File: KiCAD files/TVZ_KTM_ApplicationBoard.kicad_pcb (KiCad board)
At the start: 2 copper layers, 160 x 60 mm, 63 parts, among them SW1 EG1271A, SW2 EG1271A, SW3 EG1271A, SW4 EG1271A, U1 LM75B, U2 MCP2551-I-P, U3 MCP2551-I-P, U4 NUCLEO64-F446RE, U5 NUCLEO64-F446RE

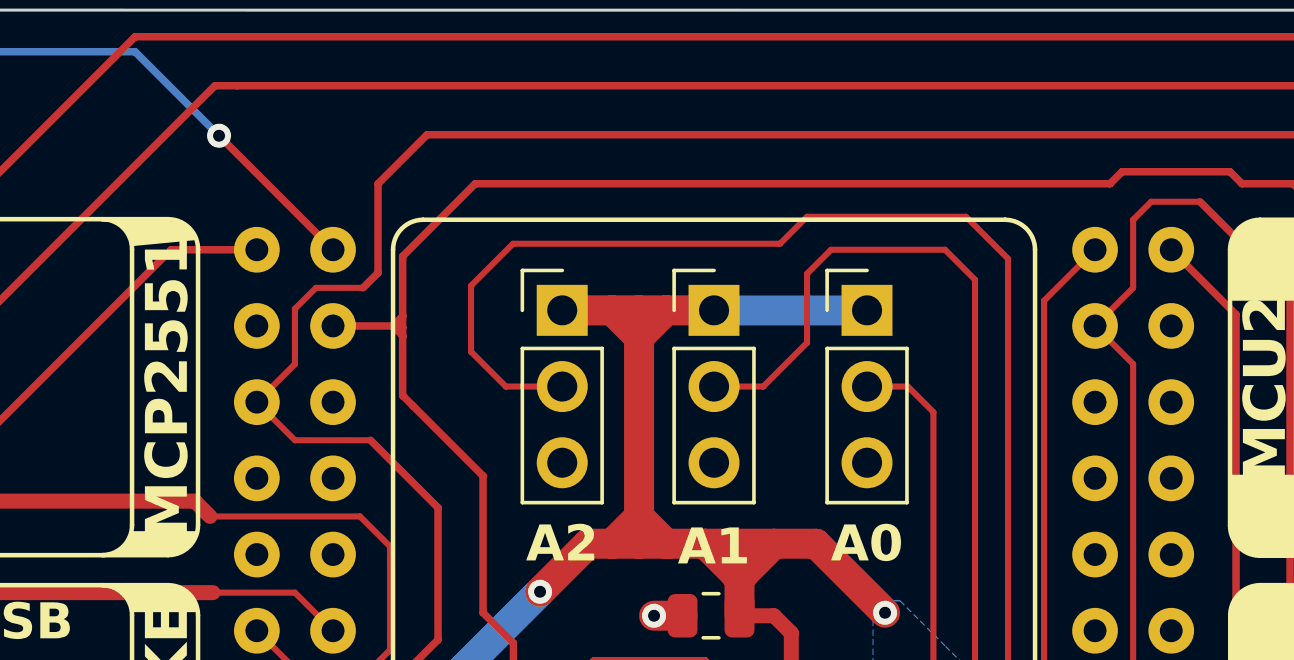
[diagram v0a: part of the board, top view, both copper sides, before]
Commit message: update
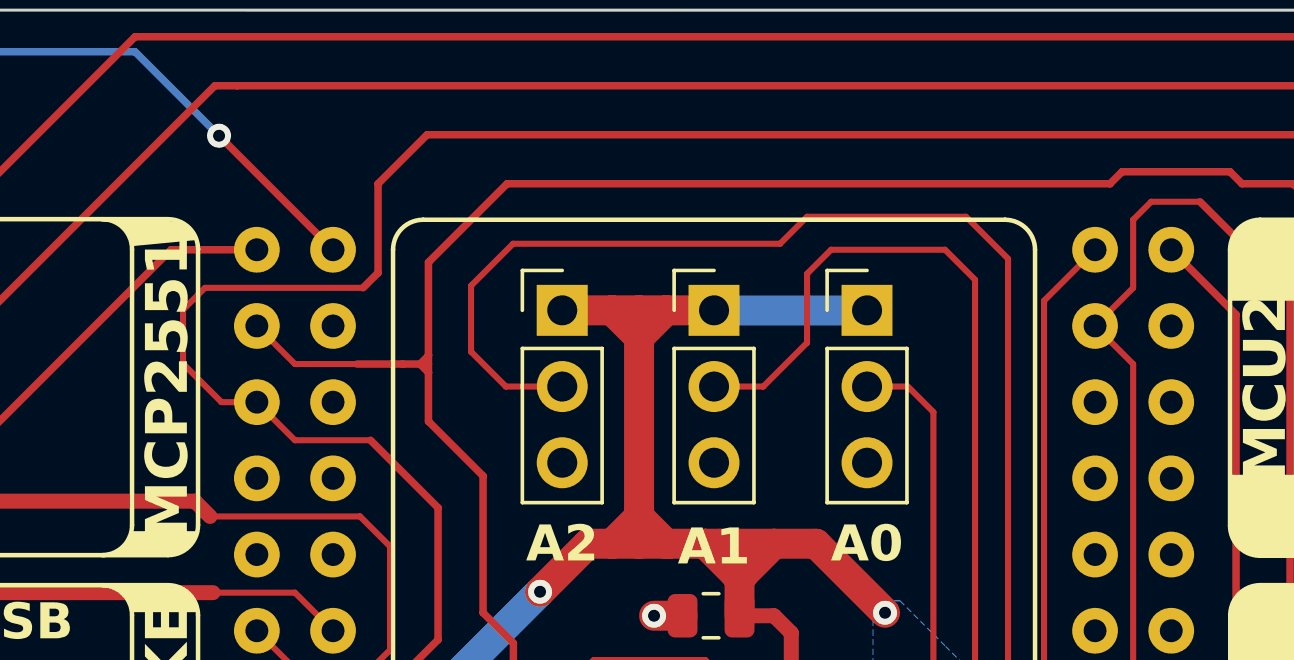
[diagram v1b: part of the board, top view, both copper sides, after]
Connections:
- U4 pad 41: unconnected-(U4-PB8-Pad41) -> I2C_SCL
- U4 pad 42: I2C_SCL -> unconnected-(U4-PC6-Pad42)
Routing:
- net I2C_SDA: track 150.3 -> 155.2 mm
- net I2C_SCL: track 147.2 -> 149.6 mm
